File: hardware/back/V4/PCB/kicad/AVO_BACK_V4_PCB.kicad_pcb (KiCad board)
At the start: 4 copper layers, 46.7 x 47.4 mm, 105 parts, among them J1 USB-C 16P, J2 BATERÍA 1S, J3 microSD DM3AT, J4 URTK1.2 (8 hilos), Q1 AO3401A, Q2 AO3401A, Q3 AO3401A, Q4 AO3401A, U1 BQ51013BRHLR, U2 BQ24072RGTR, U3 TLV75733PDBVR, U4 ESP32-S3-MINI-1U-N8, U6 USBLC6-2SC6, U7 RT9080-33GJ5, U8 DRV5032FADBZR

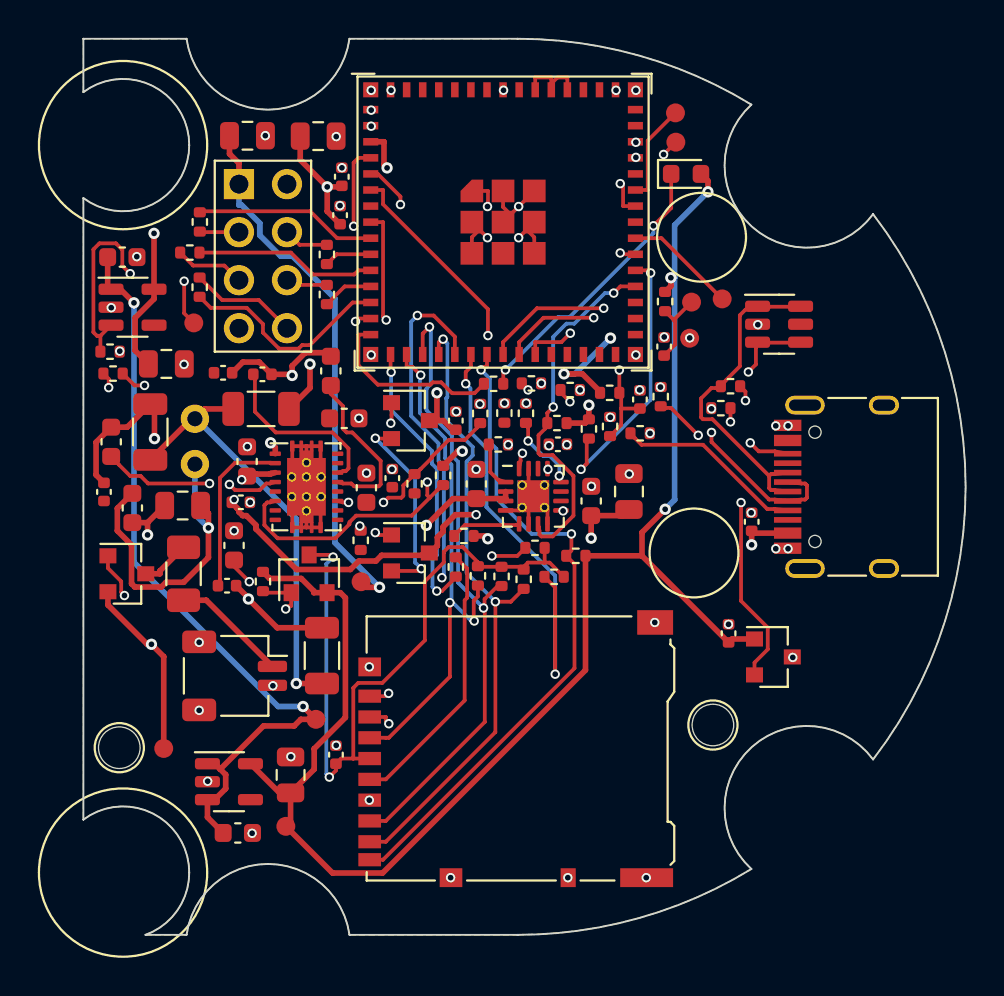
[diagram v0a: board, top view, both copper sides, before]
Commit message: PCB espalda V4: resultados de KiCad 9 de 04e2e6f (puerta: false) [skip ci]
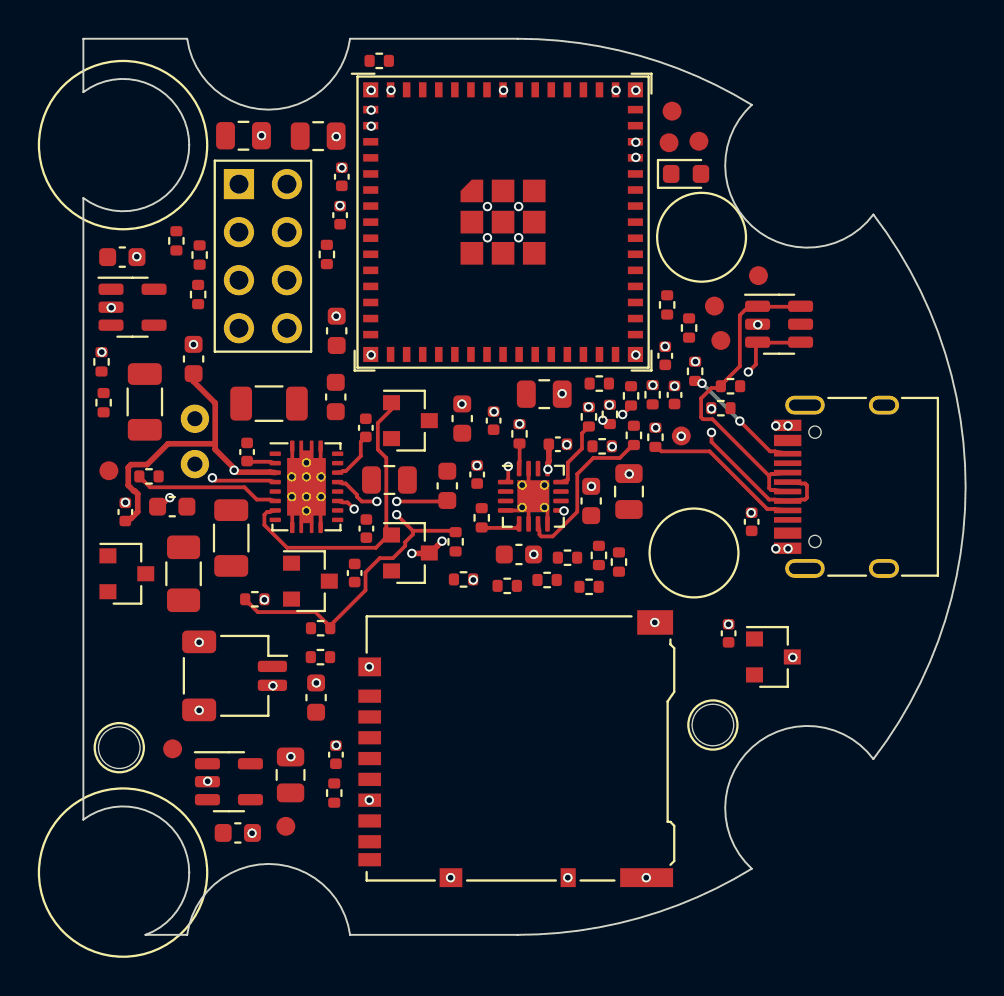
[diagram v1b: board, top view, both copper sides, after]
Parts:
- moved TP2 26.9 mm to (96.7, 81.8)
- moved TP9 22.9 mm to (99.4, 92.3)
- moved C62 20.8 mm to (90.1, 95.1)
- moved R47 17.9 mm to (79.0, 116.2), turned to 90 degrees
- moved R4 15.6 mm to (69.2, 99.5), turned to 0 degrees
- moved R2 15.5 mm to (74.8, 106.0), turned to 0 degrees
- moved TP7 15.0 mm to (67.0, 99.2)
- moved R54 14.3 mm to (81.3, 77.5)
- moved C8 14.0 mm to (80.7, 102.2)
- moved C61 12.7 mm to (74.2, 81.4)
- moved C11 12.7 mm to (80.0, 104.6), turned to 90 degrees
- moved C5 12.3 mm to (79.0, 95.2)
- moved C4 11.0 mm to (81.9, 99.6)
- moved C40 9.15 mm to (78.0, 111.2)
- moved RT1 9.06 mm to (85.8, 104.9), turned to 0 degrees
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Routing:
- net +3V3: track 136.9 -> 0.00 mm, vias 7 -> 0
- net VBAT: track 71.7 -> 0.00 mm, vias 4 -> 0
- net VSYS: track 65.0 -> 0.00 mm, vias 4 -> 0
- net QI_AC1: track 46.4 -> 0.00 mm, vias 5 -> 0
- net +3V3_SD: track 44.4 -> 0.00 mm, vias 3 -> 0
- net HALL: track 43.8 -> 0.00 mm, vias 2 -> 0
- net +3V3_ZED: track 41.9 -> 0.00 mm, vias 2 -> 0
- net SD_PWR_N: track 41.4 -> 0.00 mm, vias 2 -> 0
- net SD_D3: track 35.5 -> 0.00 mm, vias 3 -> 0
- net SD_CD: track 35.3 -> 0.00 mm, vias 2 -> 0
- net BAT_G: track 34.6 -> 0.00 mm, vias 2 -> 0
- net SD_D1: track 34.0 -> 0.00 mm, vias 2 -> 0
- net SD_D0: track 33.8 -> 0.00 mm, vias 2 -> 0
- net SD_D2: track 32.0 -> 0.00 mm, vias 4 -> 0
- net QI_AC2: track 30.5 -> 0.00 mm, vias 2 -> 0
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- removed copper zone on In2.Cu, net +3V3
- removed copper zone on B.Cu, net GND
- removed copper zone on F.Cu, net GND
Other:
- outline, holes or cut-outs redrawn

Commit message: PCB espalda V4: resultados de KiCad 9 de a08bbd6 (puerta: false) [skip ci]
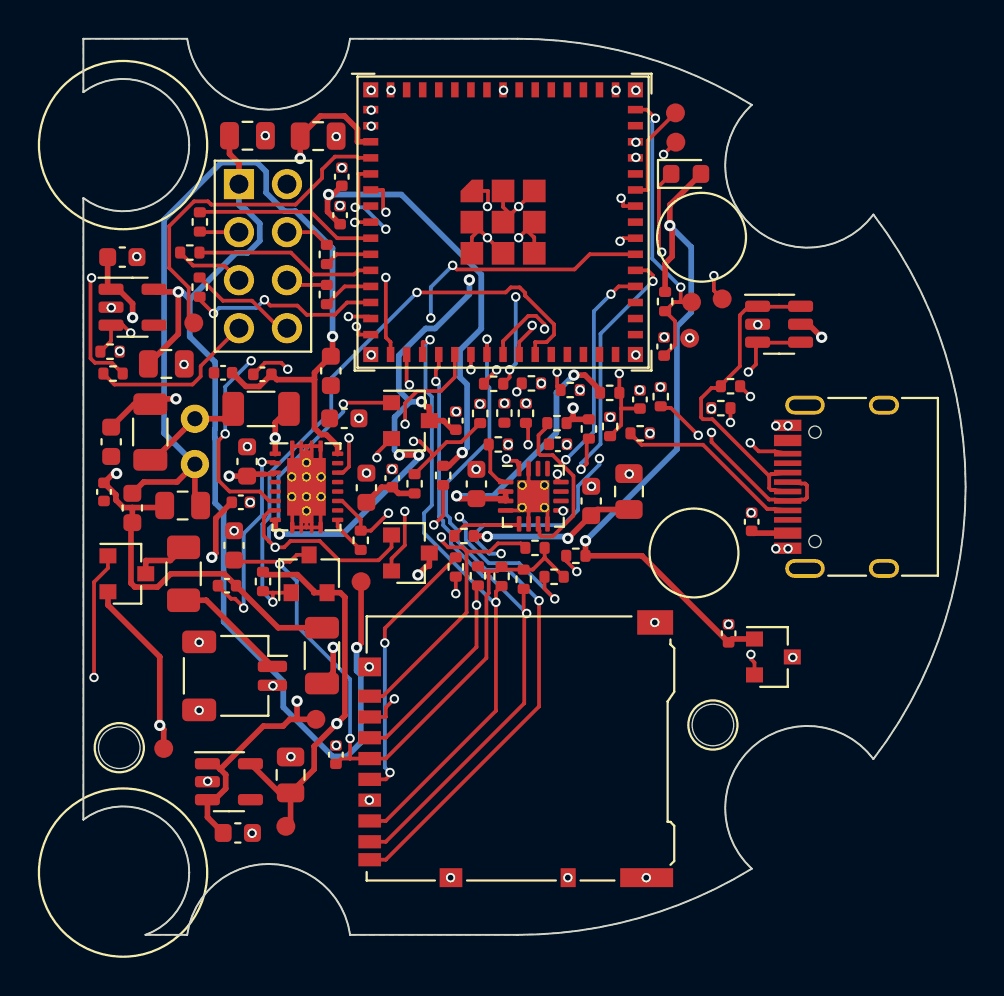
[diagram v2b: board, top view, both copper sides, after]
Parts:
- moved TP2 26.9 mm to (71.5, 91.3)
- moved TP9 22.9 mm to (80.4, 105.0)
- moved C62 20.8 mm to (74.4, 81.4)
- moved R47 17.9 mm to (91.8, 103.7), turned to 0 degrees
- moved R4 15.6 mm to (84.7, 99.4), turned to 90 degrees
- moved R2 15.5 mm to (86.7, 96.1), turned to 90 degrees
- moved TP7 15.0 mm to (70.0, 113.8)
- moved R54 14.3 mm to (71.3, 87.6)
- moved C8 14.0 mm to (66.8, 100.3)
- moved C61 12.7 mm to (70.1, 93.5)
- moved C11 12.7 mm to (73.1, 94.0), turned to 0 degrees
- moved C5 12.3 mm to (68.3, 101.1)
- moved C4 11.0 mm to (71.0, 101.0)
- moved C40 9.15 mm to (73.7, 103.1)
- moved RT1 9.06 mm to (88.0, 96.1), turned to 90 degrees
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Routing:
- net +3V3: track 0.00 -> 138.4 mm, vias 0 -> 7
- net VSYS: track 0.00 -> 60.8 mm, vias 0 -> 4
- net +3V3_ZED: track 0.00 -> 55.7 mm, vias 0 -> 2
- net BAT_G: track 0.00 -> 52.8 mm, vias 0 -> 2
- net VBAT: track 0.00 -> 50.6 mm, vias 0 -> 3
- net VBUS: track 0.00 -> 49.6 mm, vias 0 -> 6
- net QI_AC2: track 0.00 -> 49.5 mm, vias 0 -> 1
- net SD_CD: track 0.00 -> 40.0 mm, vias 0 -> 3
- net QI_CHG: track 7.71 -> 46.6 mm, vias 0 -> 5
- net QI_AC1: track 0.00 -> 38.6 mm, vias 0 -> 3
- net HALL: track 0.00 -> 38.3 mm, vias 0 -> 3
- net +3V3_SD: track 0.00 -> 37.0 mm, vias 0 -> 2
- net SD_CLK0: track 0.00 -> 35.3 mm, vias 0 -> 4
- net SD_D3: track 0.00 -> 34.8 mm, vias 0 -> 4
- net SD_D1: track 0.00 -> 33.4 mm, vias 0 -> 2
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- added copper zone on In2.Cu, net +3V3
- added copper zone on B.Cu, net GND
- added copper zone on F.Cu, net GND
